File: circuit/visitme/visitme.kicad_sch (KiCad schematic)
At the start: 15 parts, among them J5V1 Conn_01x01_Female, Q1 BC237

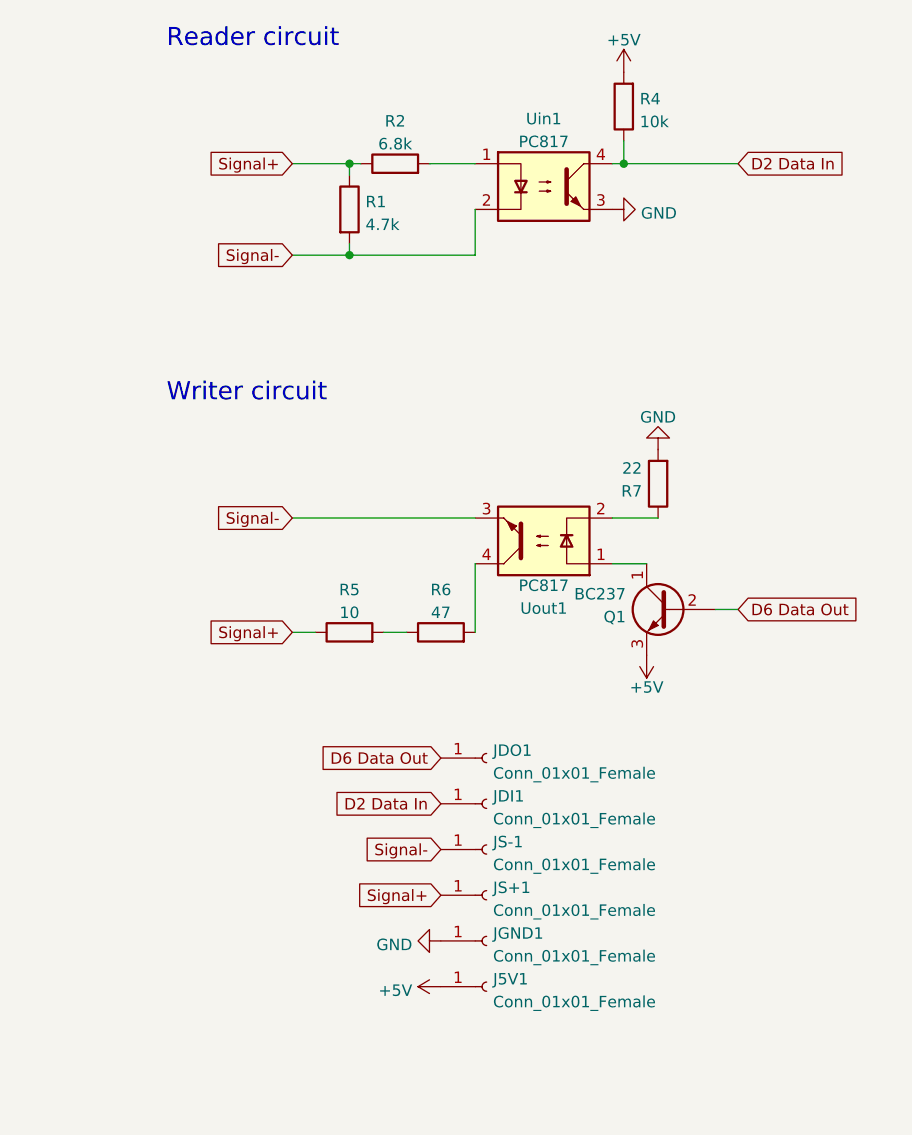
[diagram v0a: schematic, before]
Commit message: further board refinement
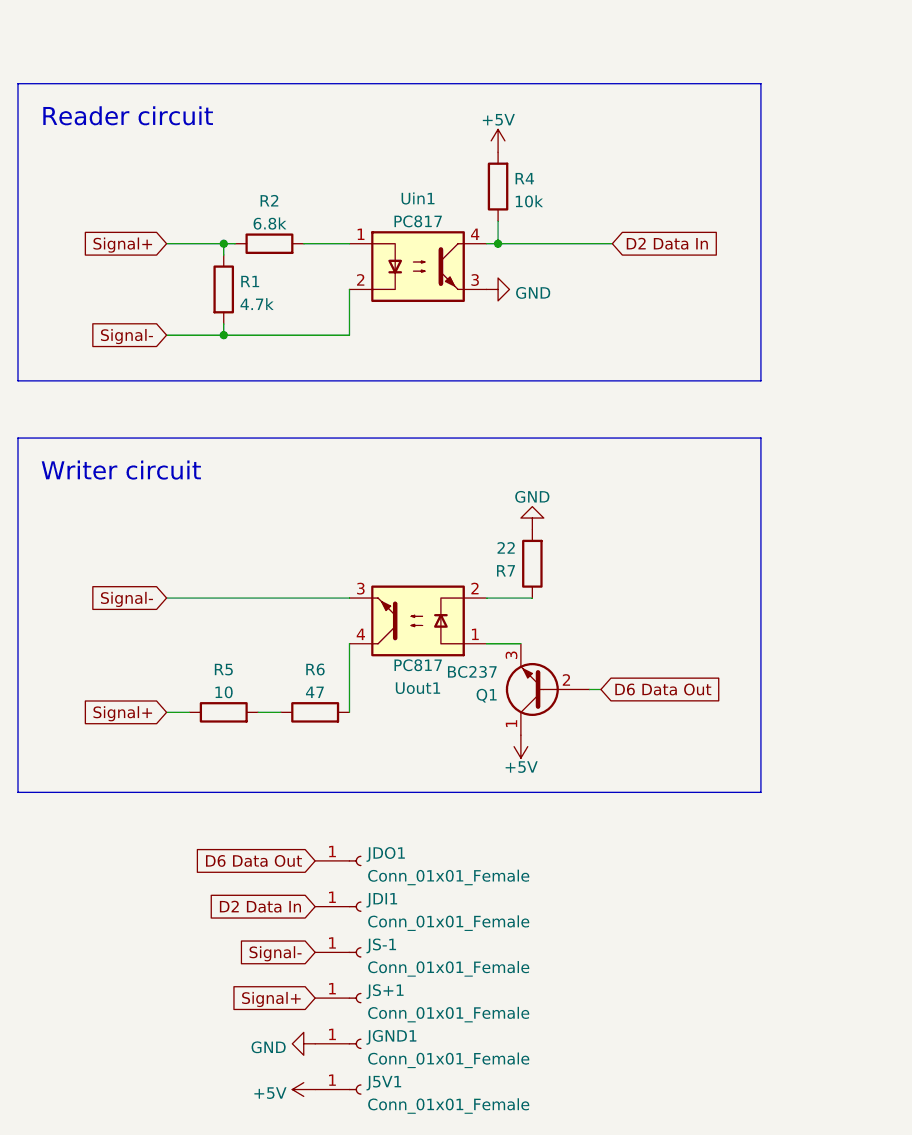
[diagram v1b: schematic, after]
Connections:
- net +5V: now also Q1.1 (C); no longer Q1.3 (E)
- net at Uout1.1: now also Q1.3 (E); no longer Q1.1 (C)
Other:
- company: (none) -> undefspace
- title: (none) -> Sebaschan Circuit
- moved on the sheet: J5V1, JDI1, JDO1, JGND1, JS+1, JS-1, Q1, R1, R2, R4, R5, R6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
